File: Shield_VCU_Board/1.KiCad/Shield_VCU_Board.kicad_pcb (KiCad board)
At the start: 2 copper layers, 250.5 x 107.1 mm, 183 parts, among them J1 Conn_02x08_Odd_Even, J10 Main_Supply, J11 Conn_01x40_Socket, J13 Conn_Molex_TouchPanel, J14 CAN_OUT, J15 Conn_01x04_Socket, J16 CAN_IN, J2 Conn_02x10_Odd_Even, J3/1 NXP3, J4 Conn_02x08_Odd_Even, J5 Conn_02x10_Odd_Even, J6 Conn_02x10_Odd_Even, J7 Button_Activation_Logic, J8 Conn_ToSpeaker, Q1 BSS138, Q2 BSS138, Q3 BSS138, Q4 BSS138, U1 AS1115-BSST, U10 TPS61165-Q1, U12 TPS54202DDC, U13 TPS54202DDC, U2 SN74LVC1G125DBV, U3 MC74HC14A, U4 TPA6205A1, U5 TLV76150DCY, U6 TLV76150DCY, U7 FT813Q, U8 TLV76133DCY, U9 TLV76133DCY

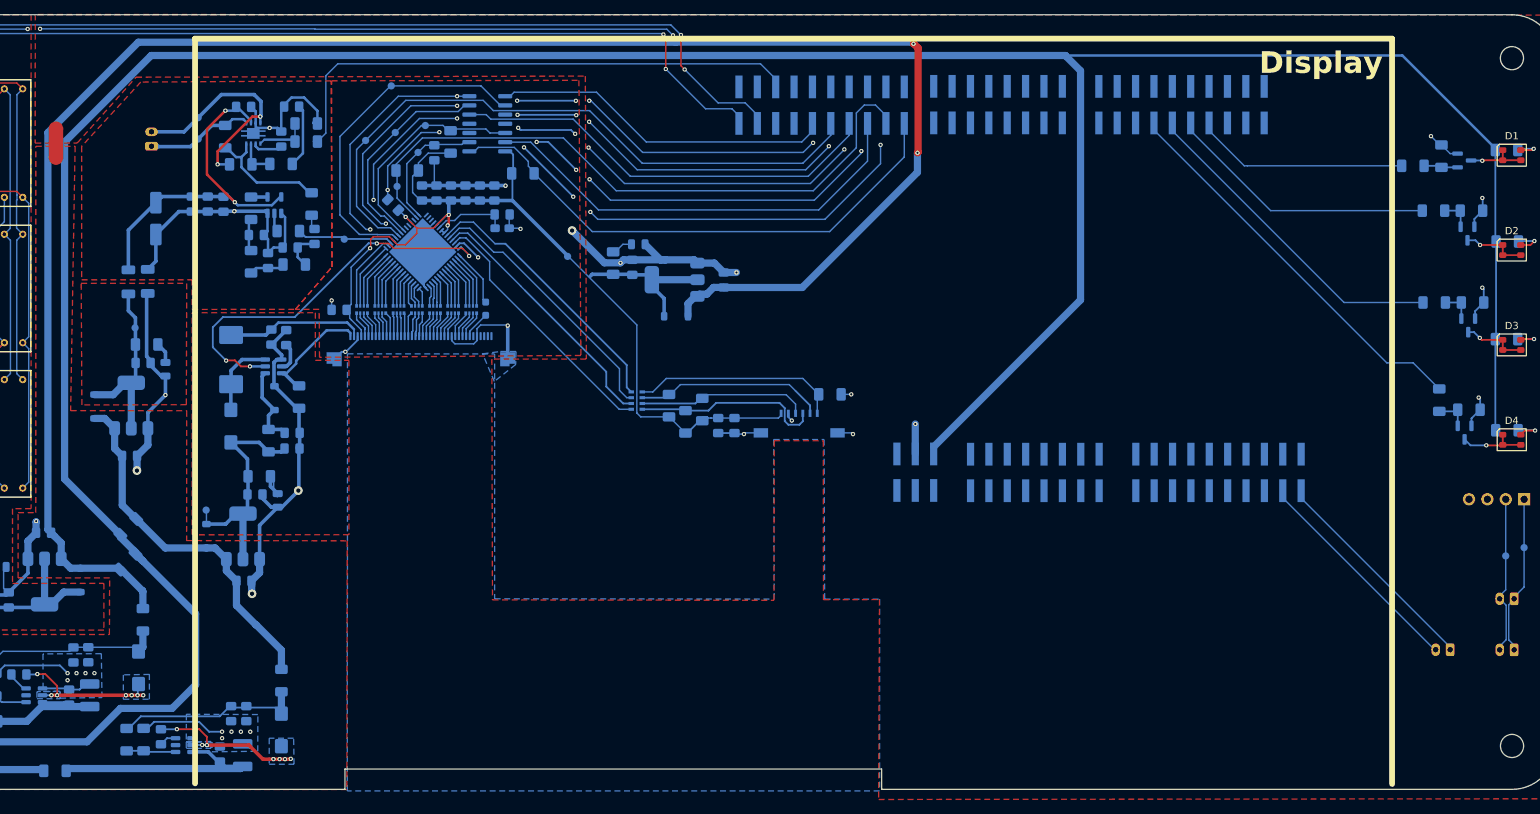
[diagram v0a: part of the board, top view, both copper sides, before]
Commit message: Check on E-plan
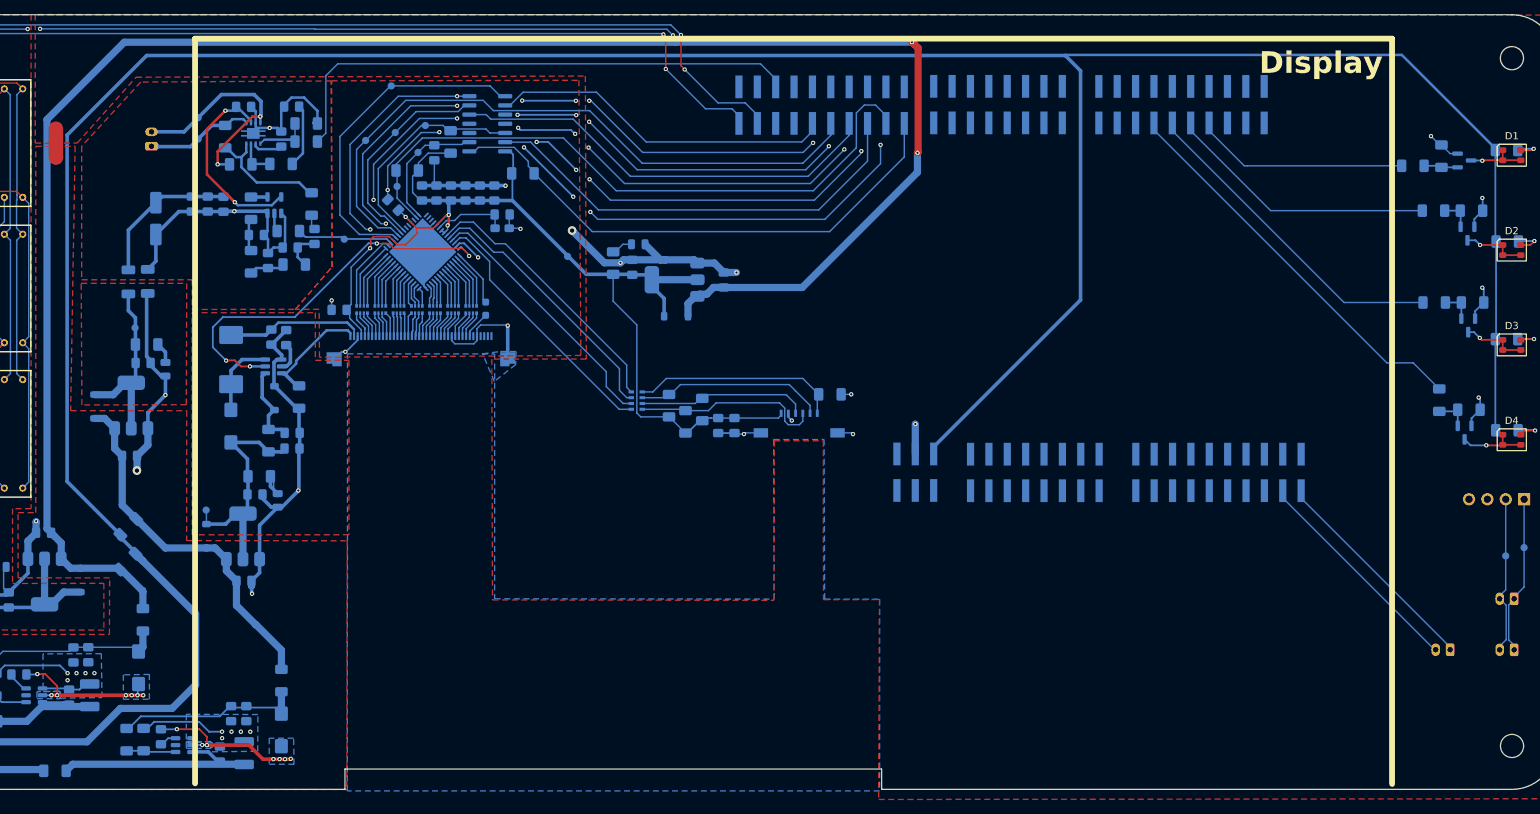
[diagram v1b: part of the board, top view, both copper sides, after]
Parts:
- moved C55 0.34 mm to (94.2, 146.1)
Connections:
- U3 pad 8: MC_SPI_SCK -> FT_T_SCK
- U3 pad 9: FT_T_SCK -> MC_SPI_SCK
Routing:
- net GND: track 804.0 -> 807.3 mm
- net Net-(U13-VIN): track 32.7 -> 29.5 mm
- net 3V3_DSPL: track 154.3 -> 153.0 mm
- net +3.7V: track 259.6 -> 260.9 mm
- net MC_SPI_SCK: track 47.3 -> 48.5 mm
